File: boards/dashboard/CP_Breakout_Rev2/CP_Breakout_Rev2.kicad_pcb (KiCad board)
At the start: 2 copper layers, 25.9 x 26.4 mm, 17 parts, among them J1 Conn_01x06, J2 Conn_01x02, J3 Conn_01x06, U1 LM2936-3.3, U2 CP2120

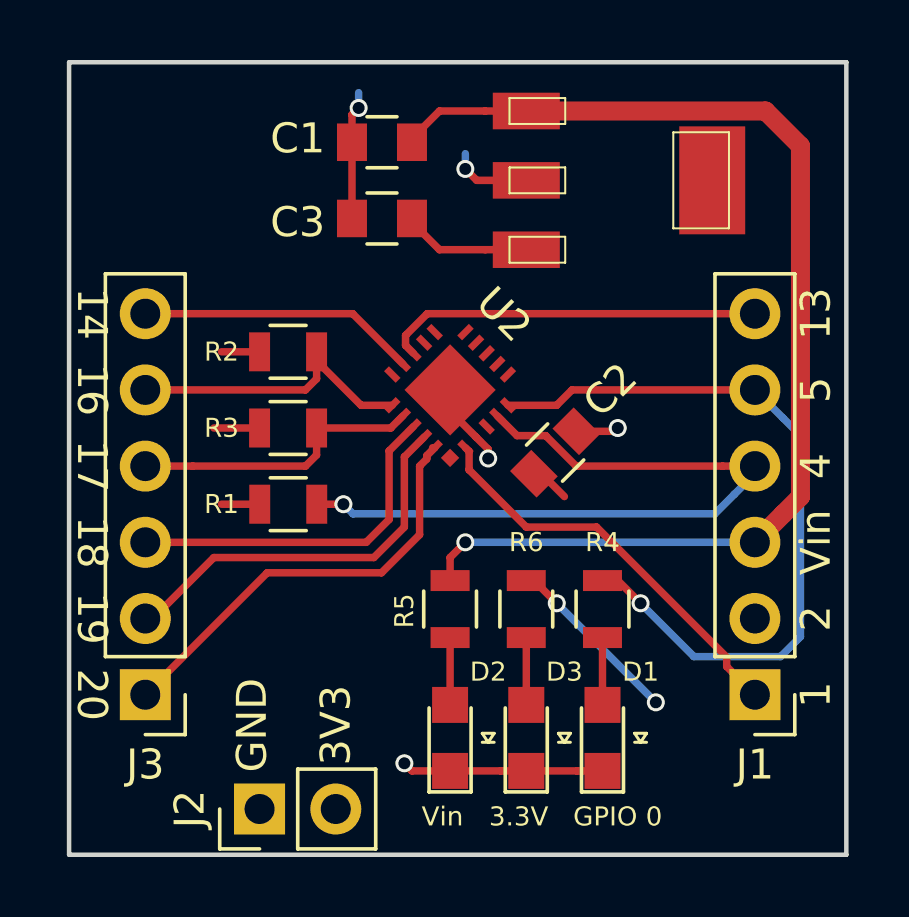
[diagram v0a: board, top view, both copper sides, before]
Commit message: Progress
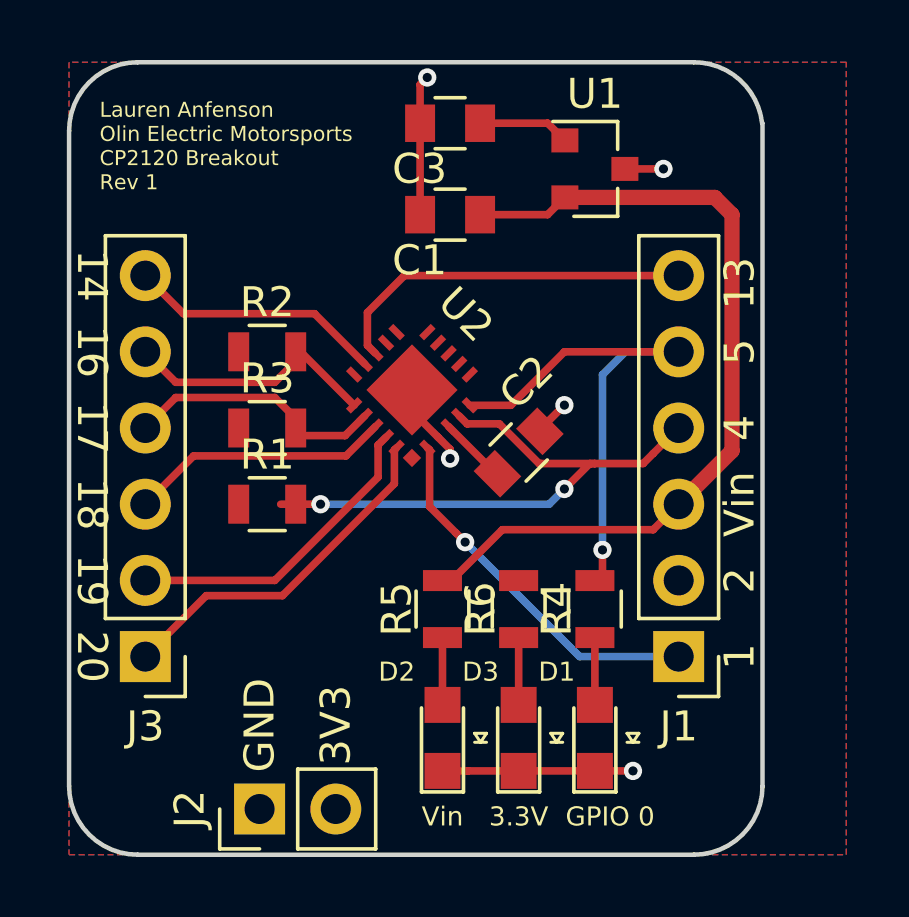
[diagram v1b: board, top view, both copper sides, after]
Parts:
- C3: value C_10uF -> C_0.1uF
- R1, R2, R3: value 4.7k -> 4.7kR
- R4, R5, R6: value R -> R_499
- U1: value LM2936-3.3 -> LM3480; footprint SparkFun-PowerIC:SOT223 -> TO_SOT_Packages_SMD:SOT-23
- moved C3 3.90 mm to (114.3, 124.5)
- moved C1 3.31 mm to (114.3, 127.5)
- moved J1 2.84 mm to (121.9, 142.2)
- moved U2 1.27 mm to (113.0, 133.3)
- moved J3 1.27 mm to (104.1, 142.2)
- moved C2 1.22 mm to (116.6, 135.4)
- moved U1 0.90 mm to (119.1, 126.0), turned to 0 degrees
- moved R1 0.70 mm to (108.2, 137.2)
- moved R2 0.70 mm to (108.2, 132.1)
- moved R3 0.70 mm to (108.2, 134.6)
- moved D3 0.25 mm to (116.6, 144.9)
- moved R6 0.25 mm to (116.6, 140.7)
- moved D1 0.25 mm to (119.1, 144.9)
- moved D2 0.25 mm to (114.0, 144.9)
- moved R4 0.25 mm to (119.1, 140.7)
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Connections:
- U1 pad 1: VCC -> +3V3
- U1 pad 2: GND -> VCC
- U1 pad 3: +3V3 -> GND
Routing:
- net VCC: track 38.9 -> 28.2 mm, vias 1 -> 0
- net +3V3: track 15.7 -> 5.34 mm, vias 2 -> 0
- net GPIO_0: track 25.2 -> 17.5 mm
- net RST: track 25.2 -> 19.5 mm, vias 1 -> 2
- net CS: track 11.9 -> 8.74 mm
- net MISO: track 14.5 -> 11.9 mm
- net MOSI: track 12.9 -> 10.6 mm
- net GND: track 17.9 -> 16.3 mm
- net SCL: track 10.2 -> 8.73 mm
- net SCLK: track 13.6 -> 12.4 mm, vias 0 -> 1
- net SDA: track 9.55 -> 8.72 mm
- net EINT: track 12.9 -> 12.4 mm
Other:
- board size 25.9 x 26.4 mm -> 23.1 x 26.4 mm
- net class Default: clearance 0.15 -> 0.1524; trace_width 0.25 -> 0.254; via_dia 0.6 -> 0.6096; via_drill 0.4 -> 0.3048
- rule trace_clearance: 0.15 -> 0.1524
- rule trace_min: 0.2 -> 0.1524
- rule via_min_drill: 0.3 -> 0.3048
- rule via_min_size: 0.4 -> 0.6096
- board text added: "Lauren Anfenson Olin Electric Motorsports CP2120 Breakout Rev 1"
